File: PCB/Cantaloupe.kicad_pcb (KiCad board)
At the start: 2 copper layers, 149.9 x 122.2 mm, 118 parts, among them J1 RGB_Out, J2 SWD, J3 Trackpad, J4 OLED, J5 Extra, J6 USB_In, J7 Split_comm_link, Q1 AO3400A, Q2 AO3400A, SW1 MX, SW10 MX, SW11 MX, SW12 MX, SW13 MX, SW14 MX, SW15 MX, SW16 MX, SW17 MX, SW18 MX, SW19 MX, SW2 MX, SW20 MX, SW21 MX, SW22 MX, SW23 MX, SW24 MX, SW25 MX, SW26 MX, SW27 MX, SW28 MX, SW29 MX, SW3 MX, SW30 MX, SW31 Encoder, SW32 Reset, SW4 MX, SW5 MX, SW6 MX, SW7 MX, SW8 MX, SW9 MX, U1 STM32F411CCU6, U2 MB85RS64, U3 SRV05-4, U4 SRV05-4, U5 W25Q128JVS, U6 XC6220B331MR-G, Y1 8MHz

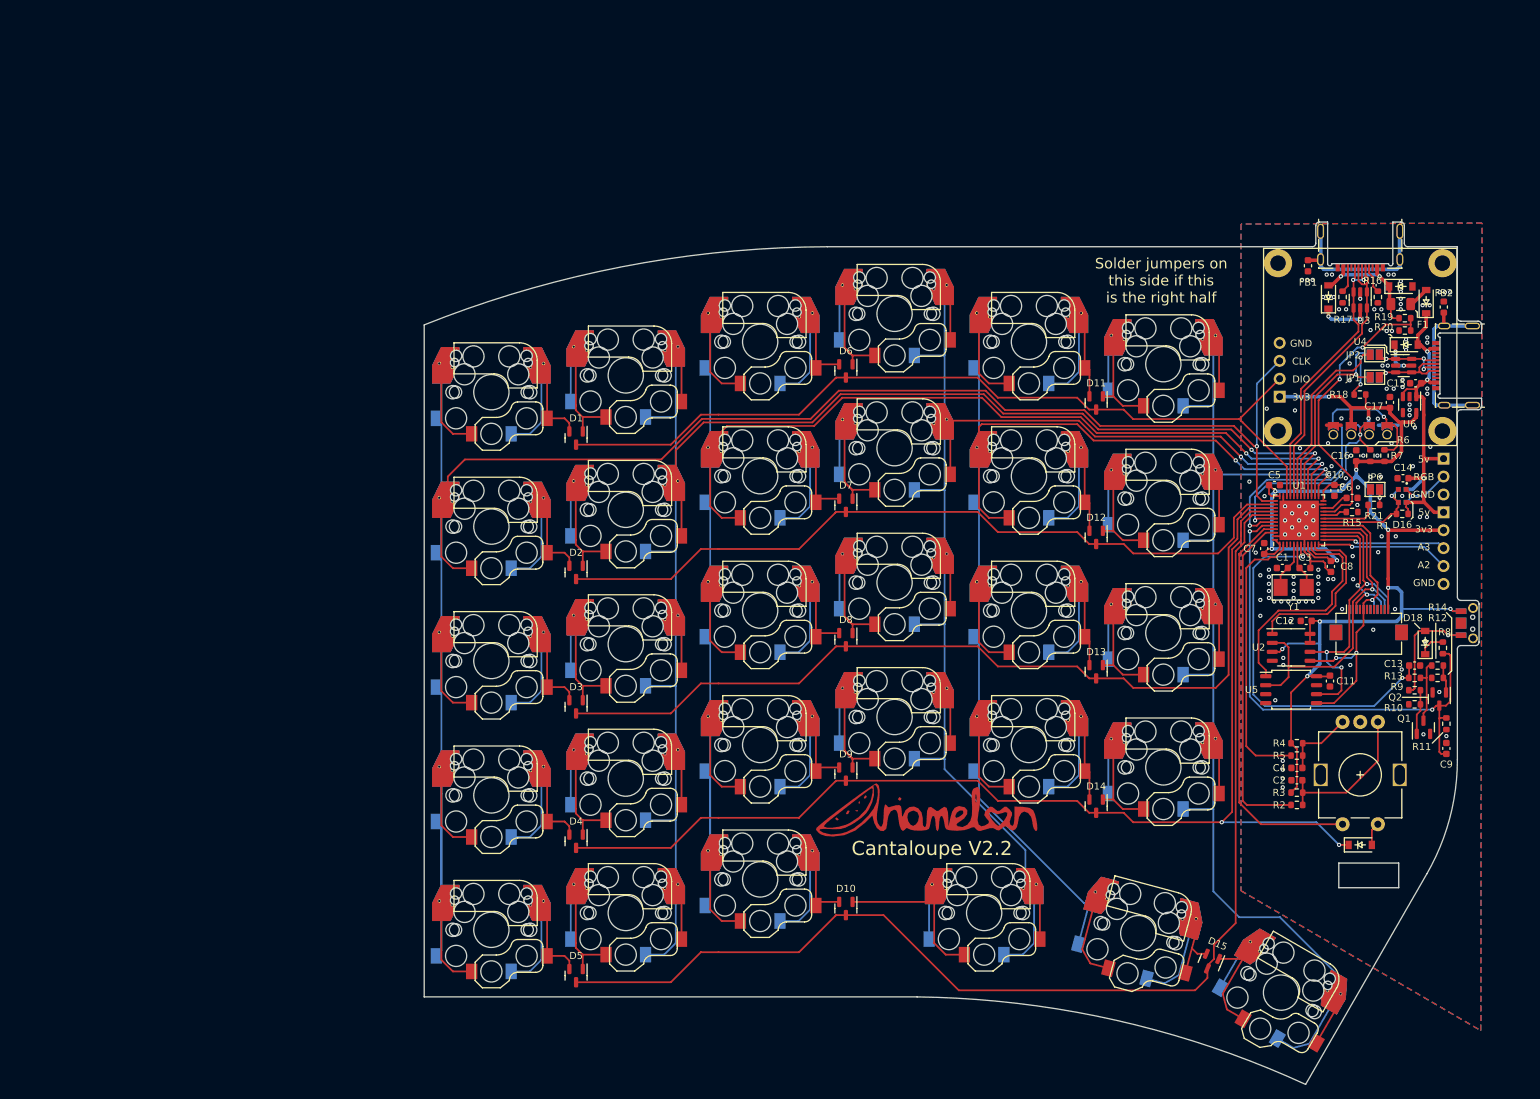
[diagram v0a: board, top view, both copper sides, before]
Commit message: INCOMPLETE V3.0 Initial Update
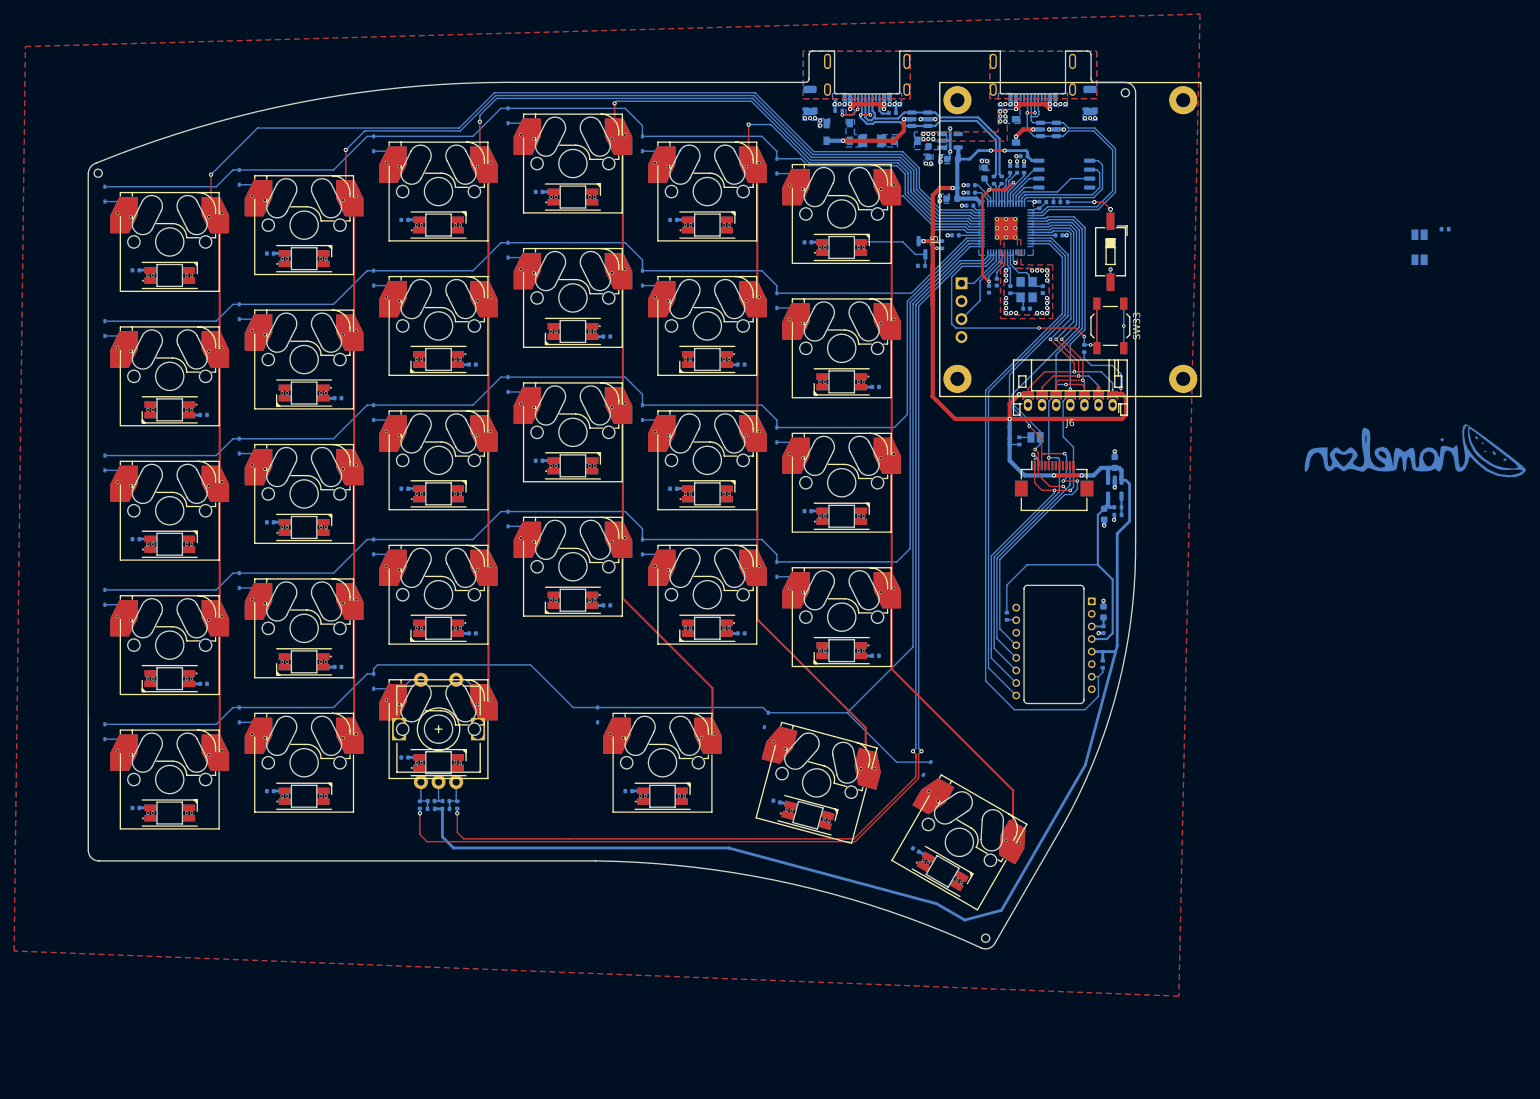
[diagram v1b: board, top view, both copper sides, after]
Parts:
- removed J7: Split_comm_link, Cantaloupe:HRO-TYPE-C-31-M-13x
- removed JP4: Link+_L, Jumper:SolderJumper-2_P1.3mm_Open_Pad1.0x1.5mm
- removed JP5: Side_L, Jumper:SolderJumper-2_P1.3mm_Open_Pad1.0x1.5mm
- removed JP6: Side_R, Jumper:SolderJumper-2_P1.3mm_Open_Pad1.0x1.5mm
- removed Q2: AO3400A, Package_TO_SOT_SMD:SOT-23
- removed R21: 10k, Resistor_SMD:R_0603_1608Metric
- added C18: 100n, Capacitor_SMD:C_0402_1005Metric, B.Cu at (138.6, 57.1)
- added C19: 4u7, Capacitor_SMD:C_0603_1608Metric, B.Cu at (153.7, 103.9)
- added C20: 100n, Capacitor_SMD:C_0402_1005Metric, B.Cu at (153.7, 106.4)
- added C21: 100n, Capacitor_SMD:C_0402_1005Metric, B.Cu at (144.6, 46.2)
- added C22: 100n, Capacitor_SMD:C_0402_1005Metric, B.Cu at (147.4, 50.5)
- added C23: 100n, Capacitor_SMD:C_0402_1005Metric, B.Cu at (132.7, 50.5)
- added C24: 1u, Capacitor_SMD:C_0603_1608Metric, B.Cu at (153.8, 90.0)
- added C25: 100n, Cantaloupe:C_0402_1005Metric, B.Cu at (16.6, 55.4)
- added C26: 100n, Cantaloupe:C_0402_1005Metric, B.Cu at (26.2, 75.9)
- added C27: 100n, Cantaloupe:C_0402_1005Metric, B.Cu at (16.6, 93.5)
- added C28: 100n, Cantaloupe:C_0402_1005Metric, B.Cu at (26.2, 114.0)
- added C29: 100n, Cantaloupe:C_0402_1005Metric, B.Cu at (16.6, 131.6)
- added C30: 100n, Cantaloupe:C_0402_1005Metric, B.Cu at (35.6, 53.0)
- added C31: 100n, Cantaloupe:C_0402_1005Metric, B.Cu at (45.2, 73.5)
- added C32: 100n, Cantaloupe:C_0402_1005Metric, B.Cu at (35.6, 91.1)
- added C33: 100n, Cantaloupe:C_0402_1005Metric, B.Cu at (45.2, 111.6)
- added C34: 100n, Cantaloupe:C_0402_1005Metric, B.Cu at (35.6, 129.2)
- added C35: 100n, Cantaloupe:C_0402_1005Metric, B.Cu at (54.7, 48.3)
- added C36: 100n, Cantaloupe:C_0402_1005Metric, B.Cu at (64.3, 68.8)
- added C37: 100n, Cantaloupe:C_0402_1005Metric, B.Cu at (54.7, 86.4)
- added C38: 100n, Cantaloupe:C_0402_1005Metric, B.Cu at (64.3, 106.9)
- added C39: 100n, Cantaloupe:C_0402_1005Metric, B.Cu at (54.7, 124.5)
- added C40: 100n, Cantaloupe:C_0402_1005Metric, B.Cu at (73.7, 44.3)
- added C41: 100n, Cantaloupe:C_0402_1005Metric, B.Cu at (83.3, 64.8)
- added C42: 100n, Cantaloupe:C_0402_1005Metric, B.Cu at (73.7, 82.4)
- added C43: 100n, Cantaloupe:C_0402_1005Metric, B.Cu at (83.3, 102.9)
- added C44: 100n, Cantaloupe:C_0402_1005Metric, B.Cu at (86.4, 129.2)
- added C45: 100n, Cantaloupe:C_0402_1005Metric, B.Cu at (92.8, 48.3)
- added C46: 100n, Cantaloupe:C_0402_1005Metric, B.Cu at (102.4, 68.8)
- added C47: 100n, Cantaloupe:C_0402_1005Metric, B.Cu at (92.8, 86.4)
- added C48: 100n, Cantaloupe:C_0402_1005Metric, B.Cu at (102.4, 106.9)
- added C49: 100n, Cantaloupe:C_0402_1005Metric, B.Cu at (107.4, 130.7)
- added C50: 100n, Cantaloupe:C_0402_1005Metric, B.Cu at (111.8, 51.5)
- added C51: 100n, Cantaloupe:C_0402_1005Metric, B.Cu at (121.4, 72.0)
- added C52: 100n, Cantaloupe:C_0402_1005Metric, B.Cu at (111.8, 89.6)
- added C53: 100n, Cantaloupe:C_0402_1005Metric, B.Cu at (121.4, 110.1)
- added C54: 100n, Cantaloupe:C_0402_1005Metric, B.Cu at (127.1, 137.6)
- added D23: 1N4148, Cantaloupe:D_SOD-323, B.Cu at (88.4, 75.6)
- added D24: 1N4148, Cantaloupe:D_SOD-323, B.Cu at (88.4, 94.6)
- added D25: 1N4148, Cantaloupe:D_SOD-323, B.Cu at (105.9, 119.1)
- added D26: 1N4148, Cantaloupe:D_SOD-323, B.Cu at (107.4, 40.7)
- added D27: 1N4148, Cantaloupe:D_SOD-323, B.Cu at (107.4, 59.7)
- added D28: 1N4148, Cantaloupe:D_SOD-323, B.Cu at (107.4, 78.8)
- added D29: 1N4148, Cantaloupe:D_SOD-323, B.Cu at (107.4, 97.8)
- added D30: 1N4148, Cantaloupe:D_SOD-323, B.Cu at (128.7, 126.0)
- added D31: SK6812MINI-E, Cantaloupe:YS-SK6812MINI-E-Flippable, B.Cu at (21.4, 56.1)
- added D32: SK6812MINI-E, Cantaloupe:YS-SK6812MINI-E-Flippable, B.Cu at (21.4, 75.2)
- added D33: SK6812MINI-E, Cantaloupe:YS-SK6812MINI-E-Flippable, B.Cu at (21.4, 94.2)
- added D34: SK6812MINI-E, Cantaloupe:YS-SK6812MINI-E-Flippable, B.Cu at (21.4, 113.3)
- added D35: SK6812MINI-E, Cantaloupe:YS-SK6812MINI-E-Flippable, B.Cu at (21.4, 132.3)
- added D36: SK6812MINI-E, Cantaloupe:YS-SK6812MINI-E-Flippable, B.Cu at (40.4, 53.8)
- added D37: SK6812MINI-E, Cantaloupe:YS-SK6812MINI-E-Flippable, B.Cu at (40.4, 72.8)
- added D38: SK6812MINI-E, Cantaloupe:YS-SK6812MINI-E-Flippable, B.Cu at (40.4, 91.9)
- added D39: SK6812MINI-E, Cantaloupe:YS-SK6812MINI-E-Flippable, B.Cu at (40.4, 110.9)
- added D40: SK6812MINI-E, Cantaloupe:YS-SK6812MINI-E-Flippable, B.Cu at (40.4, 130.0)
- added D41: SK6812MINI-E, Cantaloupe:YS-SK6812MINI-E-Flippable, B.Cu at (59.5, 49.0)
- added D42: SK6812MINI-E, Cantaloupe:YS-SK6812MINI-E-Flippable, B.Cu at (59.5, 68.1)
- added D43: SK6812MINI-E, Cantaloupe:YS-SK6812MINI-E-Flippable, B.Cu at (59.5, 87.1)
- added D44: SK6812MINI-E, Cantaloupe:YS-SK6812MINI-E-Flippable, B.Cu at (59.5, 106.2)
- added D45: SK6812MINI-E, Cantaloupe:YS-SK6812MINI-E-Flippable, B.Cu at (59.5, 125.2)
- added D46: SK6812MINI-E, Cantaloupe:YS-SK6812MINI-E-Flippable, B.Cu at (78.5, 45.0)
- added D47: SK6812MINI-E, Cantaloupe:YS-SK6812MINI-E-Flippable, B.Cu at (78.5, 64.1)
- added D48: SK6812MINI-E, Cantaloupe:YS-SK6812MINI-E-Flippable, B.Cu at (78.5, 83.1)
- added D49: SK6812MINI-E, Cantaloupe:YS-SK6812MINI-E-Flippable, B.Cu at (78.5, 102.2)
- added D50: SK6812MINI-E, Cantaloupe:YS-SK6812MINI-E-Flippable, B.Cu at (91.2, 130.0)
- added D51: SK6812MINI-E, Cantaloupe:YS-SK6812MINI-E-Flippable, B.Cu at (97.6, 49.0)
- added D52: SK6812MINI-E, Cantaloupe:YS-SK6812MINI-E-Flippable, B.Cu at (97.6, 68.1)
- added D53: SK6812MINI-E, Cantaloupe:YS-SK6812MINI-E-Flippable, B.Cu at (97.6, 87.1)
- added D54: SK6812MINI-E, Cantaloupe:YS-SK6812MINI-E-Flippable, B.Cu at (97.6, 106.2)
- added D55: SK6812MINI-E, Cantaloupe:YS-SK6812MINI-E-Flippable, B.Cu at (111.8, 132.7)
- added D56: SK6812MINI-E, Cantaloupe:YS-SK6812MINI-E-Flippable, B.Cu at (116.6, 52.2)
- added D57: SK6812MINI-E, Cantaloupe:YS-SK6812MINI-E-Flippable, B.Cu at (116.6, 71.2)
- added D58: SK6812MINI-E, Cantaloupe:YS-SK6812MINI-E-Flippable, B.Cu at (116.6, 90.3)
- added D59: SK6812MINI-E, Cantaloupe:YS-SK6812MINI-E-Flippable, B.Cu at (116.6, 109.3)
- added D60: SK6812MINI-E, Cantaloupe:YS-SK6812MINI-E-Flippable, B.Cu at (130.9, 140.6)
- added D67: B5819W SL, Cantaloupe:D_SOD-123, B.Cu at (141.3, 35.7)
- added D68: SMF5.0A, Cantaloupe:D_SOD-123, B.Cu at (116.1, 34.6)
- added D69: B5819W SL, Cantaloupe:D_SOD-123, B.Cu at (116.1, 37.1)
- added D70: B5819W SL, Cantaloupe:D_SOD-123, B.Cu at (125.7, 37.1)
- added H1: Tooling Hole, Cantaloupe:JLC Tooling Hole, F.Cu at (156.8, 30.3)
- added H2: Tooling Hole, Cantaloupe:JLC Tooling Hole, F.Cu at (11.2, 41.7)
- added H3: Tooling Hole, Cantaloupe:JLC Tooling Hole, F.Cu at (137.0, 150.1)
- added SW33: Reset, Cantaloupe:SW_SPST_TL3342-Dual, F.Cu at (154.7, 63.3)
- added U7: AP2127K-ADJ, Package_TO_SOT_SMD:SOT-23-5, B.Cu at (155.3, 86.3)
- A1, F1, Q1, U4: moved to B.Cu
- C1: value 20p -> 10n; footprint Capacitor_SMD:C_0603_1608Metric -> Capacitor_SMD:C_0402_1005Metric; moved to B.Cu
- C10, C13, C14: footprint Capacitor_SMD:C_0603_1608Metric -> Capacitor_SMD:C_0402_1005Metric; moved to B.Cu
- C11, C12, C5: value 100n -> 1u; moved to B.Cu
- C15, C16, C17, C9: value 10u -> 100n; footprint Capacitor_SMD:C_0603_1608Metric -> Capacitor_SMD:C_0402_1005Metric; moved to B.Cu
- C2: value 100n -> 10n; footprint Capacitor_SMD:C_0603_1608Metric -> Capacitor_SMD:C_0402_1005Metric; moved to B.Cu
- C3: value 20p -> 4u7; moved to B.Cu
- C4: value 100n -> 4u7; moved to B.Cu
- C6: value 4.7u -> 100n; footprint Capacitor_SMD:C_0603_1608Metric -> Capacitor_SMD:C_0402_1005Metric; moved to B.Cu
- C7, C8: value 100n -> 22p; footprint Capacitor_SMD:C_0603_1608Metric -> Capacitor_SMD:C_0402_1005Metric; moved to B.Cu
- D1, D10, D11, D12, D13, D14, D15, D2, D3, D4, D5, D6, D7, D8, D9: value D_Dual_CommonCathode_AAK_Split_Small -> 1N4148; footprint Package_TO_SOT_SMD:SOT-23 -> Cantaloupe:D_SOD-323; moved to B.Cu
- D16: value WS2812C-2020 -> 1N4148; footprint Cantaloupe:LED_WS2812-2020_Flippable -> Cantaloupe:D_SOD-323; moved to B.Cu
- D17, D18: value D -> 1N4148; footprint Cantaloupe:D_SOD-123 -> Cantaloupe:D_SOD-323; moved to B.Cu
- D19, D21, D22: value B5819W SL -> 1N4148; footprint Cantaloupe:D_SOD-123 -> Cantaloupe:D_SOD-323; moved to B.Cu
- D20: value SMF5.0A -> 1N4148; footprint Cantaloupe:D_SOD-123 -> Cantaloupe:D_SOD-323; moved to B.Cu
- FB1, FB2: value GZ1608D110TF -> 60R@100MHz; footprint Inductor_SMD:L_0603_1608Metric -> Inductor_SMD:L_1206_3216Metric; moved to B.Cu
- J1: value RGB_Out -> SWD; footprint Cantaloupe:PinHeader_1x03_P2.54mm_Vertical_Silkless -> Connector_PinHeader_2.54mm:PinHeader_1x04_P2.54mm_Vertical
- J2: value SWD -> USB_In; footprint Cantaloupe:PinHeader_1x04_P2.54mm_Vertical_SIlkless -> Cantaloupe:HRO-TYPE-C-31-M-13x
- J3: value Trackpad -> Split_comm_link; footprint Cantaloupe:Hirose_FH12-12S-0.5SH_1x12-1MP_P0.50mm_Horizontal_Flippable -> Cantaloupe:HRO-TYPE-C-31-M-13x; moved to B.Cu
- J4: value OLED -> Trackpad; footprint Cantaloupe:OLED_0.96_SSD1306_128x64_Flippable_Reversepads -> Cantaloupe:Hirose_FH12-12S-0.5SH_1x12-1MP_P0.50mm_Horizontal_Flippable; moved to B.Cu
- J5: value Extra -> OLED; footprint Cantaloupe:PinHeader_1x05_P2.54mm_Vertical_Silkless -> Cantaloupe:OLED_1.5_SSD1315_128x128_NoPins
- J6: value USB_In -> OLED_PH; footprint Cantaloupe:HRO-TYPE-C-31-M-13x -> Cantaloupe:JST_PH_S7B-PH-K_1x07_P2.00mm_Horizontal-Dual
- JP1: value Link-_R -> Side_L; moved to B.Cu
- JP2: value Link+_R -> Side_R; moved to B.Cu
- JP3: value Link-_L -> MISO_Pullup
- R1, R16, R17: value 5k1 -> 10k; footprint Resistor_SMD:R_0603_1608Metric -> Resistor_SMD:R_0402_1005Metric; moved to B.Cu
- R10: value 10k -> 1k; footprint Resistor_SMD:R_0603_1608Metric -> Resistor_SMD:R_0402_1005Metric; moved to B.Cu
- R11: value 1M -> 5k1; footprint Resistor_SMD:R_0603_1608Metric -> Resistor_SMD:R_0402_1005Metric; moved to B.Cu
- R12: value 10k -> 5k1; footprint Resistor_SMD:R_0603_1608Metric -> Resistor_SMD:R_0402_1005Metric; moved to B.Cu
- R13: value 100 -> 10k; footprint Resistor_SMD:R_0603_1608Metric -> Resistor_SMD:R_0402_1005Metric; moved to B.Cu
- R14: value 100k -> 39; footprint Resistor_SMD:R_0603_1608Metric -> Resistor_SMD:R_0402_1005Metric; moved to B.Cu
- R15: value 100k -> 10k; footprint Resistor_SMD:R_0603_1608Metric -> Resistor_SMD:R_0402_1005Metric; moved to B.Cu
- R18: value 10k -> 15k; footprint Resistor_SMD:R_0603_1608Metric -> Resistor_SMD:R_0402_1005Metric; moved to B.Cu
- R19: value 5.1k -> 10k; footprint Resistor_SMD:R_0603_1608Metric -> Resistor_SMD:R_0402_1005Metric; moved to B.Cu
- R2, R20, R3, R4, R5: footprint Resistor_SMD:R_0603_1608Metric -> Resistor_SMD:R_0402_1005Metric; moved to B.Cu
- R6, R7: value 4k7 -> 1k; footprint Resistor_SMD:R_0603_1608Metric -> Resistor_SMD:R_0402_1005Metric; moved to B.Cu
- R8: value 100k -> 27; footprint Resistor_SMD:R_0603_1608Metric -> Resistor_SMD:R_0402_1005Metric; moved to B.Cu
- R9: value 1k -> 27; footprint Resistor_SMD:R_0603_1608Metric -> Resistor_SMD:R_0402_1005Metric; moved to B.Cu
- SW1, SW10, SW11, SW12, SW13, SW14, SW15, SW16, SW17, SW18, SW19, SW2, SW20, SW21, SW22, SW23, SW24, SW25, SW26, SW27, SW28, SW29, SW3, SW30, SW4, SW5, SW6, SW7, SW8, SW9: value MX -> CPG151101S11; footprint Cantaloupe:MX_Choc-1U-Hotswap-Dual -> Cantaloupe:MX_1U-Hotswap-Dual; moved to B.Cu
- SW32: value Reset -> USB Boot; footprint Cantaloupe:Switch_TS24ZJ_Flippable -> Cantaloupe:SW_DIP_SPSTx01_Slide_6.7x4.1mm_W8.61mm_P2.54mm_LowProfile-Dual; moved to B.Cu
- U1: value STM32F411CCU6 -> AP2127K-3.3; footprint Package_DFN_QFN:QFN-48-1EP_7x7mm_P0.5mm_EP5.6x5.6mm -> Package_TO_SOT_SMD:SOT-23-5; moved to B.Cu
- U2: value MB85RS64 -> W25Q128JVS; footprint Package_SO:SSOP-8_3.9x5.05mm_P1.27mm -> Package_SO:SOIC-8_5.23x5.23mm_P1.27mm; moved to B.Cu
- U3: value SRV05-4 -> RP2040; footprint Package_TO_SOT_SMD:SOT-23-6 -> Cantaloupe:QFN-56-1EP_7x7mm_P0.4mm_EP3.2x3.2mm_ThermalVias; moved to B.Cu
- U5: value W25Q128JVS -> SRV05-4; footprint Package_SO:SOIC-8_5.275x5.275mm_P1.27mm -> Package_TO_SOT_SMD:SOT-23-6; moved to B.Cu
- U6: value XC6220B331MR-G -> PMW3360DM-T2QU; footprint Package_TO_SOT_SMD:SOT-23-5 -> Cantaloupe:IC_PMW3360DM-T2QU; moved to B.Cu
- Y1: value 8MHz -> 12MHz; footprint Crystal:Crystal_SMD_5032-2Pin_5.0x3.2mm -> Crystal:Crystal_SMD_3225-4Pin_3.2x2.5mm; moved to B.Cu
- moved D17 147.3 mm to (69.3, 52.6), turned to -90 degrees
- moved R1 145.2 mm to (56.8, 131.2), turned to -90 degrees
- moved D16 137.7 mm to (69.3, 33.5)
- moved D18 135.0 mm to (69.3, 71.6), turned to -90 degrees
- moved SW31 130.8 mm to (59.5, 120.5), turned to 0 degrees
- moved D19 129.7 mm to (69.3, 90.7), turned to -90 degrees
- moved D20 129.0 mm to (82.0, 118.4), turned to -90 degrees
- moved C1 125.1 mm to (58.4, 130.7), turned to 180 degrees
- moved D15 125.1 mm to (50.3, 113.7), turned to -90 degrees
- moved R2 122.7 mm to (58.4, 131.8)
- moved R11 122.3 mm to (116.2, 32.8), turned to 0 degrees
- moved C2 120.6 mm to (60.5, 130.7)
- moved R3 120.6 mm to (60.5, 131.8), turned to 0 degrees
- moved R4 119.3 mm to (62.1, 131.2), turned to 90 degrees
- moved D22 111.1 mm to (88.4, 56.5), turned to -90 degrees
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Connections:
- C1 pad 2: HSE_IN -> Net-(C1-Pad2)
- C10 pad 2: +3V3 -> +1V1
- C11 pad 2: +3V3 -> +1V1
- C13 pad 2: NRST -> +3V3
- C14 pad 2: +5V -> +3V3
- C15 pad 2: +5V -> +3V3
- C3 pad 2: HSE_OUT -> +5V
- C4 pad 2: Net-(C4-Pad2) -> +3V3
- C5 pad 1: GND -> +3V3
- C5 pad 2: +3V3 -> GND
- C6 pad 2: Net-(C6-Pad2) -> +3V3
- C7 pad 2: +3V3 -> Net-(U3-XIN)
- C8 pad 2: +3V3 -> Net-(C8-Pad2)
- C9 pad 1: BOOT0 -> GND
- C9 pad 2: GND -> +1V1
- D1 pad 1: Net-(D1-Pad1) -> /MCU/ROW0
- D1 pad 2: Net-(D1-Pad2) -> Net-(D1-A)
- D10 pad 1: Net-(D10-Pad1) -> /MCU/ROW4
- D10 pad 2: Net-(D10-Pad2) -> Net-(D10-A)
- D11 pad 1: Net-(D11-Pad1) -> /MCU/ROW0
- D11 pad 2: Net-(D11-Pad2) -> Net-(D11-A)
- D12 pad 1: Net-(D12-Pad1) -> /MCU/ROW1
- D12 pad 2: Net-(D12-Pad2) -> Net-(D12-A)
- D13 pad 1: Net-(D13-Pad1) -> /MCU/ROW2
- D13 pad 2: Net-(D13-Pad2) -> Net-(D13-A)
- D14 pad 1: Net-(D14-Pad1) -> /MCU/ROW3
- D14 pad 2: Net-(D14-Pad2) -> Net-(D14-A)
- D15 pad 1: Net-(D15-Pad1) -> /MCU/ROW4
- D15 pad 2: Net-(D15-Pad2) -> Net-(D15-A)
- D16 pad 1: Net-(D16-Pad1) -> /MCU/ROW0
- D16 pad 2: GND -> Net-(D16-A)
- D17 pad 1: ROW3 -> /MCU/ROW1
- D17 pad 2: Net-(D17-Pad2) -> Net-(D17-A)
- D18 pad 1: Net-(D18-Pad1) -> /MCU/ROW2
- D18 pad 2: Net-(D18-Pad2) -> Net-(D18-A)
- D19 pad 1: Net-(D19-Pad1) -> /MCU/ROW3
- D19 pad 2: +5V -> Net-(D19-A)
- D2 pad 1: Net-(D2-Pad1) -> /MCU/ROW1
- D2 pad 2: Net-(D2-Pad2) -> Net-(D2-A)
- D20 pad 1: VBUS -> /MCU/ROW4
- D20 pad 2: GND -> Net-(D20-A)
- D21 pad 1: Net-(D21-Pad1) -> /MCU/ROW0
- D21 pad 2: VBUS -> Net-(D21-A)
- D22 pad 1: +5V -> /MCU/ROW1
- D22 pad 2: Net-(D22-Pad2) -> Net-(D22-A)
- D3 pad 1: Net-(D3-Pad1) -> /MCU/ROW2
- D3 pad 2: Net-(D3-Pad2) -> Net-(D3-A)
- D4 pad 1: Net-(D4-Pad1) -> /MCU/ROW3
- D4 pad 2: Net-(D4-Pad2) -> Net-(D4-A)
- D5 pad 1: Net-(D5-Pad1) -> /MCU/ROW4
- D5 pad 2: Net-(D5-Pad2) -> Net-(D5-A)
- D6 pad 1: Net-(D6-Pad1) -> /MCU/ROW0
- D6 pad 2: Net-(D6-Pad2) -> Net-(D6-A)
- D7 pad 1: Net-(D7-Pad1) -> /MCU/ROW1
- D7 pad 2: Net-(D7-Pad2) -> Net-(D7-A)
- D8 pad 1: Net-(D8-Pad1) -> /MCU/ROW2
- D8 pad 2: Net-(D8-Pad2) -> Net-(D8-A)
- D9 pad 1: Net-(D9-Pad1) -> /MCU/ROW3
- D9 pad 2: Net-(D9-Pad2) -> Net-(D9-A)
- F1 pad 1: Net-(D22-Pad2) -> Net-(D70-A)
- FB1 pad 1: GND -> Net-(J2-SHIELD)
- FB1 pad 2: Net-(FB1-Pad2) -> GND
- FB2 pad 1: GND -> Net-(J3-SHIELD)
- FB2 pad 2: Net-(FB2-Pad2) -> GND
- J1 pad 1: +5V -> Net-(J1-Pin_1)
- J1 pad 2: Net-(D16-Pad1) -> GND
- J1 pad 3: GND -> Net-(J1-Pin_3)
- J4 pad 1: GND -> /Comms/SCK
- J4 pad 2: +3V3 -> /Comms/MISO
- J4 pad 3: SCL -> /Comms/SS_TB
- J4 pad 4: SDA -> unconnected-(J4-Pin_4-Pad4)
- JP1 pad 1: TX -> +3V3
- JP1 pad 2: Link- -> Net-(JP1-B)
- JP2 pad 1: RX -> GND
- JP2 pad 2: Link+ -> Net-(JP1-B)
- JP3 pad 1: RX -> Net-(JP3-A)
- JP3 pad 2: Link- -> /Comms/MISO
- Q1 pad 1: Net-(Q1-Pad1) -> +3V3
- Q1 pad 2: GND -> Net-(Q1-S)
- Q1 pad 3: Net-(Q1-Pad3) -> /MCU/RGB
- R1 pad 1: +5V -> Net-(C1-Pad2)
- R1 pad 2: LED -> /MCU/ROTA
- R10 pad 1: GND -> Net-(JP1-B)
- R10 pad 2: Net-(Q1-Pad1) -> /MCU/Side
- R11 pad 1: BOOT0 -> GND
- R11 pad 2: GND -> Net-(J2-CC1)
- R12 pad 1: Net-(Q2-Pad1) -> GND
- R12 pad 2: Net-(Q1-Pad3) -> Net-(J2-CC2)
- R13 pad 1: Net-(Q1-Pad3) -> /Comms/~{RST}_TB
- R13 pad 2: NRST -> +3V3
- R14 pad 1: Net-(Q2-Pad1) -> Net-(U6-LED_P)
- R14 pad 2: GND -> +2V
- R15 pad 1: BOOT1 -> Net-(JP3-A)
- R15 pad 2: GND -> +3V3
- R16 pad 1: GND -> Net-(U7-ADJ)
- R16 pad 2: Net-(J6-PadA5) -> GND
- R17 pad 1: GND -> Net-(SW33-B)
- R17 pad 2: Net-(J6-PadB5) -> +3V3
- R18 pad 1: +3V3 -> +2V
- R18 pad 2: RX -> Net-(U7-ADJ)
- R19 pad 1: VBUS -> Net-(Q1-S)
- R19 pad 2: PLUGGED -> +3V3
- R2 pad 1: ROT_A -> Net-(C1-Pad2)
- R2 pad 2: Net-(C2-Pad2) -> +3V3
- R20 pad 1: PLUGGED -> /MCU/RGB
- R20 pad 2: GND -> +5V
- R3 pad 1: Net-(C2-Pad2) -> +3V3
- R3 pad 2: +3V3 -> Net-(C2-Pad2)
- R4 pad 1: +3V3 -> /MCU/ROTB
- R4 pad 2: Net-(C4-Pad2) -> Net-(C2-Pad2)
- R5 pad 1: Net-(C4-Pad2) -> Net-(U2-~{CS})
- R5 pad 2: ROT_B -> +3V3
- R6 pad 1: SCL -> Net-(R6-Pad1)
- R6 pad 2: +3V3 -> Net-(U2-~{CS})
- R7 pad 1: SDA -> Net-(C8-Pad2)
- R7 pad 2: +3V3 -> Net-(U3-XOUT)
- R8 pad 1: BOOT0 -> /Comms/D+
- R8 pad 2: Net-(D18-Pad1) -> Net-(U3-USB_DP)
- R9 pad 1: Net-(D18-Pad2) -> /Comms/D-
- R9 pad 2: Net-(Q1-Pad1) -> Net-(U3-USB_DM)
- SW1 pad 1: COL0 -> Net-(D1-A)
- SW1 pad 2: Net-(D1-Pad2) -> /MCU/COL0
- SW10 pad 1: Net-(D5-Pad1) -> Net-(D10-A)
- SW10 pad 2: COL1 -> /MCU/COL1
- SW11 pad 1: COL2 -> Net-(D11-A)
- SW11 pad 2: Net-(D6-Pad2) -> /MCU/COL2
- SW12 pad 1: COL2 -> Net-(D12-A)
- SW12 pad 2: Net-(D7-Pad2) -> /MCU/COL2
- SW13 pad 1: COL2 -> Net-(D13-A)
- SW13 pad 2: Net-(D8-Pad2) -> /MCU/COL2
- SW14 pad 1: COL2 -> Net-(D14-A)
- SW14 pad 2: Net-(D9-Pad2) -> /MCU/COL2
- SW15 pad 1: COL2 -> Net-(D15-A)
- SW15 pad 2: Net-(D10-Pad2) -> /MCU/COL2
- SW16 pad 1: Net-(D6-Pad1) -> Net-(D16-A)
- SW16 pad 2: COL3 -> /MCU/COL3
- SW17 pad 1: Net-(D7-Pad1) -> Net-(D17-A)
- SW17 pad 2: COL3 -> /MCU/COL3
- SW18 pad 1: Net-(D8-Pad1) -> Net-(D18-A)
- SW18 pad 2: COL3 -> /MCU/COL3
- SW19 pad 1: Net-(D9-Pad1) -> Net-(D19-A)
- SW19 pad 2: COL3 -> /MCU/COL3
- SW2 pad 1: COL0 -> Net-(D2-A)
- SW2 pad 2: Net-(D2-Pad2) -> /MCU/COL0
- SW20 pad 1: Net-(D10-Pad1) -> Net-(D20-A)
- SW20 pad 2: COL3 -> /MCU/COL3
- SW21 pad 1: COL4 -> Net-(D21-A)
- SW21 pad 2: Net-(D11-Pad2) -> /MCU/COL4
- SW22 pad 1: COL4 -> Net-(D22-A)
- SW22 pad 2: Net-(D12-Pad2) -> /MCU/COL4
- SW23 pad 1: COL4 -> Net-(D23-A)
- SW23 pad 2: Net-(D13-Pad2) -> /MCU/COL4
- SW24 pad 1: COL4 -> Net-(D24-A)
- SW24 pad 2: Net-(D14-Pad2) -> /MCU/COL4
- SW25 pad 1: COL4 -> Net-(D25-A)
- SW25 pad 2: Net-(D15-Pad2) -> /MCU/COL4
- SW26 pad 1: Net-(D11-Pad1) -> Net-(D26-A)
- SW26 pad 2: COL5 -> /MCU/COL5
- SW27 pad 1: Net-(D12-Pad1) -> Net-(D27-A)
- SW27 pad 2: COL5 -> /MCU/COL5
- SW28 pad 1: Net-(D13-Pad1) -> Net-(D28-A)
- SW28 pad 2: COL5 -> /MCU/COL5
- SW29 pad 1: Net-(D14-Pad1) -> Net-(D29-A)
- SW29 pad 2: COL5 -> /MCU/COL5
- SW3 pad 1: COL0 -> Net-(D3-A)
- SW3 pad 2: Net-(D3-Pad2) -> /MCU/COL0
- SW30 pad 1: Net-(D15-Pad1) -> Net-(D30-A)
- SW30 pad 2: COL5 -> /MCU/COL5
- SW31 pad A: Net-(C2-Pad2) -> Net-(C1-Pad2)
- SW31 pad B: Net-(C4-Pad2) -> Net-(C2-Pad2)
- SW31 pad S1: COLROT -> /MCU/COL2
- SW31 pad S2: Net-(D17-Pad2) -> Net-(D15-A)
- SW32 pad 1: +3V3 -> Net-(R6-Pad1)
- SW32 pad 2: Net-(D18-Pad2) -> GND
- SW4 pad 1: COL0 -> Net-(D4-A)
- SW4 pad 2: Net-(D4-Pad2) -> /MCU/COL0
- SW5 pad 1: COL0 -> Net-(D5-A)
- SW5 pad 2: Net-(D5-Pad2) -> /MCU/COL0
- SW6 pad 1: Net-(D1-Pad1) -> Net-(D6-A)
- SW6 pad 2: COL1 -> /MCU/COL1
- SW7 pad 1: Net-(D2-Pad1) -> Net-(D7-A)
- SW7 pad 2: COL1 -> /MCU/COL1
- SW8 pad 1: Net-(D3-Pad1) -> Net-(D8-A)
- SW8 pad 2: COL1 -> /MCU/COL1
- SW9 pad 1: Net-(D4-Pad1) -> Net-(D9-A)
- SW9 pad 2: COL1 -> /MCU/COL1
- U1 pad 1: +3V3 -> +5V
- U1 pad 2: ROT_B -> GND
- U1 pad 3: unconnected-(U1-Pad3) -> +5V
- U1 pad 5: HSE_IN -> +3V3
- U2 pad 1: SS_EEPROM -> Net-(U2-~{CS})
- U2 pad 2: MISO -> Net-(U2-DO(IO1))
- U2 pad 3: +3V3 -> Net-(U2-IO2)
- U2 pad 5: MOSI -> Net-(U2-DI(IO0))
- U2 pad 6: SCK -> Net-(U2-CLK)
- U2 pad 7: +3V3 -> Net-(U2-IO3)
- U3 pad 1: D- -> +3V3
- U3 pad 2: GND -> /Comms/RX
- U3 pad 3: D+ -> /Comms/TX
- U3 pad 4: D+ -> /Comms/SCK
- U3 pad 5: Net-(D21-Pad1) -> /Comms/MOSI
- U3 pad 6: D- -> /Comms/MISO
- U4 pad 1: Link+ -> /Comms/D+
- U4 pad 3: Link- -> /Comms/D-
- U4 pad 4: Link- -> /Comms/D-
- U4 pad 5: Net-(D19-Pad1) -> Net-(D69-K)
- U4 pad 6: Link+ -> /Comms/D+
- U5 pad 1: SS_Flash -> /Comms/TX
- U5 pad 2: MISO -> GND
- U5 pad 3: unconnected-(U5-Pad3) -> /Comms/RX
- U5 pad 4: GND -> /Comms/RX
- U5 pad 5: MOSI -> Net-(D67-K)
- U5 pad 6: SCK -> /Comms/TX
- U6 pad 1: +5V -> unconnected-(U6-NC-Pad1)
- U6 pad 2: GND -> unconnected-(U6-NC-Pad2)
- U6 pad 3: +5V -> Net-(U6-VDDPIX)
- U6 pad 4: unconnected-(U6-Pad4) -> +2V
- Y1 pad 1: HSE_IN -> Net-(U3-XIN)
- Y1 pad 2: HSE_OUT -> GND
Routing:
- net COL0: track 308.9 -> 0.00 mm, vias 1 -> 0
- net COL2: track 257.7 -> 0.00 mm, vias 2 -> 0
- net COL1: track 248.1 -> 0.00 mm, vias 2 -> 0
- net COL4: track 215.5 -> 0.00 mm, vias 2 -> 0
- net COL3: track 210.3 -> 0.00 mm, vias 2 -> 0
- net /MCU/COL0: track 0.00 -> 203.4 mm, vias 0 -> 1
- net /MCU/ROW4: track 0.00 -> 201.7 mm
- net /MCU/COL1: track 0.00 -> 183.9 mm, vias 0 -> 1
- net COL5: track 181.7 -> 0.00 mm, vias 1 -> 0
- net /MCU/ROW3: track 0.00 -> 172.5 mm
- net ROW4: track 169.6 -> 0.00 mm
- net /MCU/COL2: track 0.00 -> 166.9 mm, vias 0 -> 1
- net ROW3: track 166.4 -> 0.00 mm, vias 2 -> 0
- net /MCU/ROTA: track 0.00 -> 159.6 mm, vias 0 -> 2
- net /MCU/COL3: track 0.00 -> 154.6 mm, vias 0 -> 1
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- added copper zone on B.Cu, net +3V3
- added copper zone on B.Cu, net +5V
- added copper zone on F.Cu, net +5V
- added copper zone on B.Cu, net Net-(D70-A)
- added copper zone on B.Cu, net Net-(J2-SHIELD)
- added copper zone on F.Cu, net Net-(J2-SHIELD)
- added copper zone on B.Cu, net Net-(J3-SHIELD)
- added copper zone on F.Cu, net Net-(J3-SHIELD)
- added copper zone on B.Cu, net VBUS
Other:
- board size 149.9 x 122.2 mm -> 148.5 x 127.3 mm
- board text added: "Cantaloupe V3.0"
- board text added: "OLED"
- board text removed: "3v3"
- board text removed: "5v"
- board text removed: "A2"
- board text removed: "A3"
- board text removed: "CLK"
- board text removed: "Cantaloupe V2.2"
- board text removed: "DIO"
- board text removed: "GND"
- board text removed: "RGB"
- board text removed: "Solder jumpers on this side if this is the left half"
- board text removed: "Solder jumpers on this side if this is the right half"
